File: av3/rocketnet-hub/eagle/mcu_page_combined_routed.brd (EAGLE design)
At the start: 112.7 x 76.3 mm, 446 parts, among them J1 ROCKETNET-CONNECTOR-16M, J10 UART Header, J11 I2C Header, J12 BOOT1 Jumper, J13 PGOOD Jumper, J14 ROCKETNET-UMBILICAL-18, J15 Auxiliary Header, J16 Auxiliary Header, J17 Auxiliary Header, J18 Auxiliary Header, J19 Auxiliary Header, J2 ROCKETNET-CONNECTOR-16M, J20 Auxiliary Header, J21 Auxiliary Header, J22 Debug Header, J3 ROCKETNET-CONNECTOR-16M, J4 ROCKETNET-CONNECTOR-16M, J5 BOOT0 Jumper, J6 ROCKETNET-CONNECTOR-16M, J7 ROCKETNET-CONNECTOR-16M, J8 ROCKETNET-CONNECTOR-16M, J9 ROCKETNET-BATTERY-14, Q2 FDS6680ASOIC8, Q3 FDS6680ASOIC8, Q4 FDS6680ASOIC8, Q5 SIS412DNSOP-8, Q6 BSS138W-7-F, Q7 SIS412DNSOP-8, T1 BSS84, T10 ALT4532, T11 ALT4532, T12 ALT4532, T13 ALT4532, T14 ALT4532, T15 ALT4532, T16 ALT4532, T17 ALT4532, T18 ALT4532, T19 BSS84, T2 NDS335N, T20 NDS335N, T3 ALT4532, T4 ALT4532, T5 ALT4532, T6 ALT4532, T7 ALT4532, T8 ALT4532, T9 ALT4532, U1 STM32F407V100-PIN_QFP, U10 TPS2420QFN-16, U11 TPS2420QFN-16, U12 TPS2420QFN-16, U13 TPS2420QFN-16, U14 MAX4734ETC+, U15 MAX4734ETC+, U2 BQ24725QFN-20, U3 SN65220DBV, U4 KS8999, U5 LTM8023, U6 MIC37101-2.1YM, U7 TPS2420QFN-16, U8 TPS2420QFN-16, U9 TPS2420QFN-16

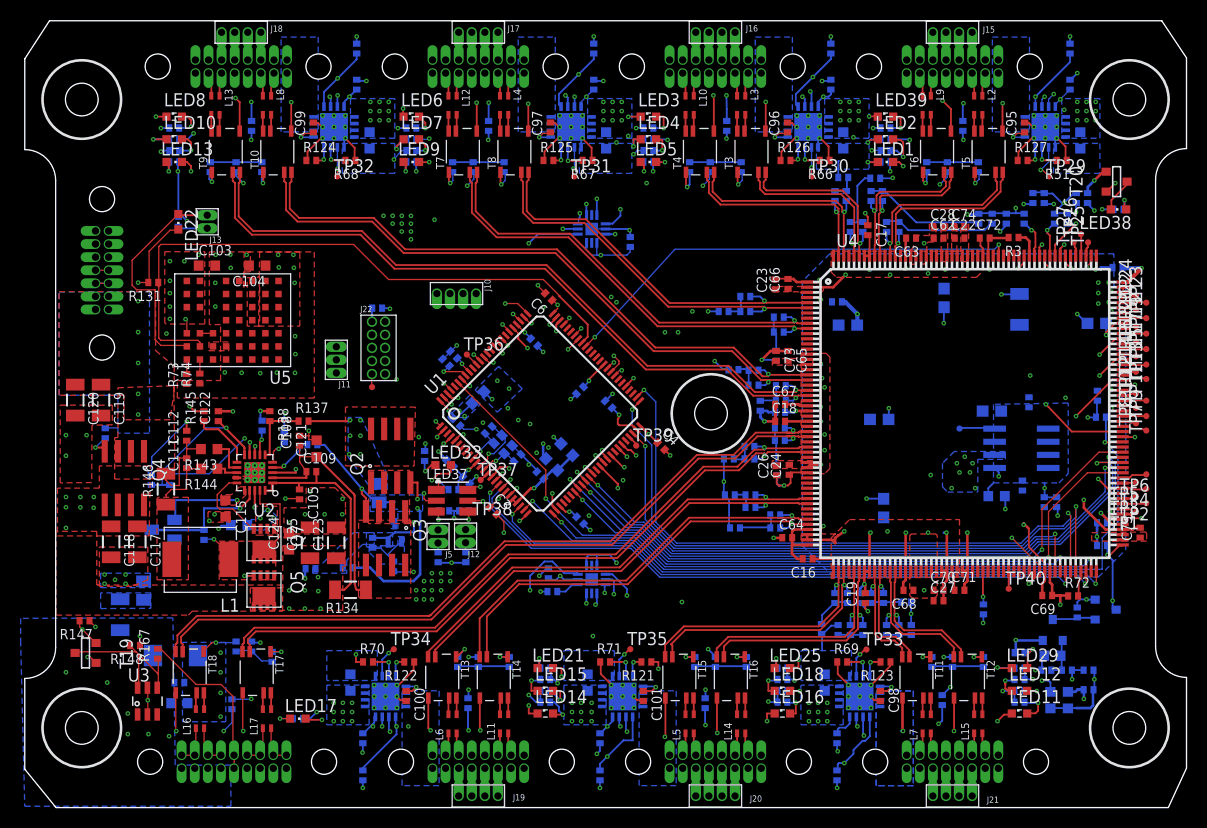
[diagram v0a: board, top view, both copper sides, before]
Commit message: fixed all drc issues
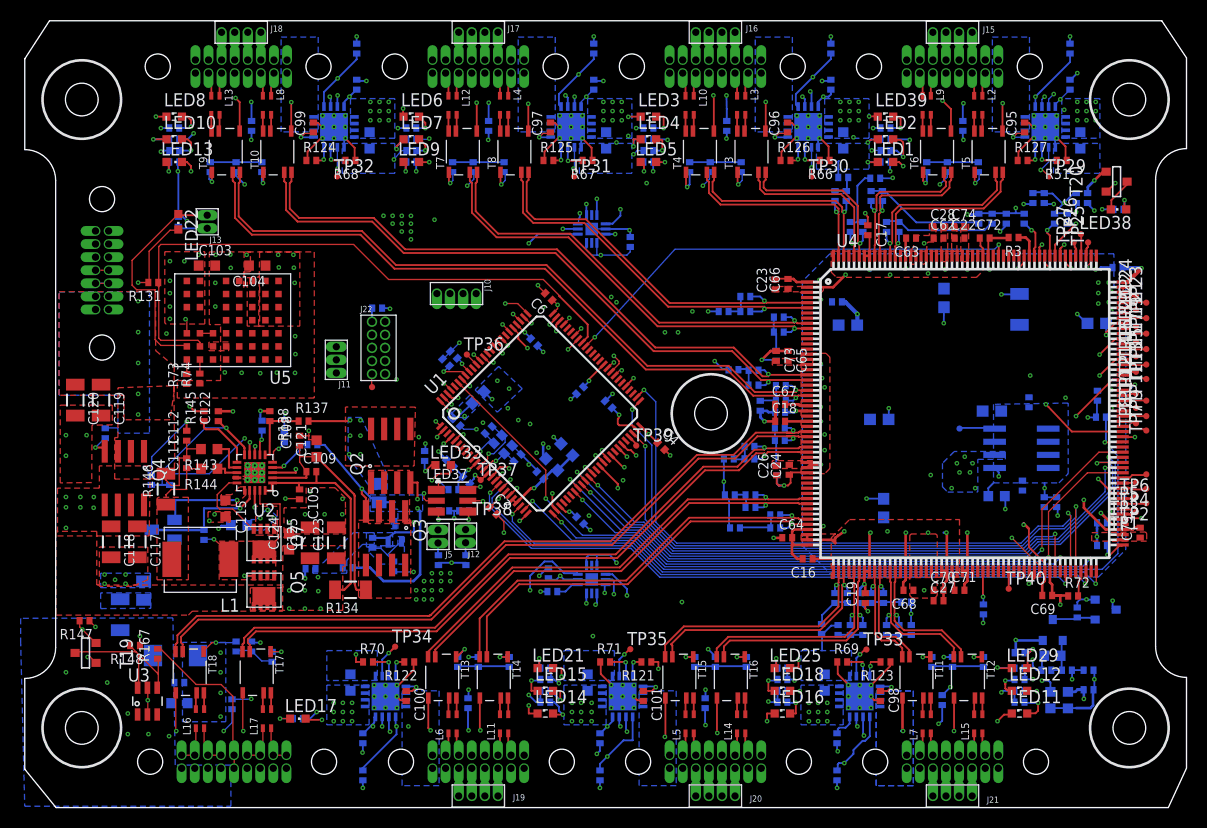
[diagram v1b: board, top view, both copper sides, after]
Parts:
- moved TP34 0.28 mm to (35.9, 15.5)
- moved R64 0.28 mm to (40.1, 23.9)
- moved R150 0.28 mm to (42.8, 23.9)
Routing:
- net VDDIO_IN: track 42.8 -> 44.5 mm
- net NODE4_IMON_IN: track 40.5 -> 42.2 mm
- net +3V3: track 146.1 -> 146.7 mm
- net GND: track 254.2 -> 254.7 mm
